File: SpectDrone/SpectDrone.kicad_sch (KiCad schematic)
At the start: 128 parts, among them J1 Conn_02x03_Counter_Clockwise, J1-1 Conn_01x04_Male, J1-2 Conn_01x04_Male, J1V0-1 Conn_01x01_Male, J2 GPS, J3 Barrel_Jack, J3V1-1 Conn_01x01_Male, J3V3 Conn_01x01_Male, J4 BME280, J5 RFShield_OnePiece, J5-1 BNO055-1, J5-2 BNO055-2, J5V3-1 Conn_01x01_Male, J5V3-2 Conn_01x01_Male, Q1 FDN340P, Q2 FDN340P, SW0 SW_Push, SW1 SW_Push, SW10 SW_Push, SW2 SW_Push, SW3 SW_Push, SW4 SW_Push, SW5 SW_Push, SW6 SW_Push, SW7 SW_Push, SW8 SW_Push, SW9 SW_Push, U1 C12666MA, U10 TXS0102DCUR, U11 PCA9306DC, U12 AD799x, U2 C12666MA, U3 LM7805_TO220, U4 MCP112-450E/TO, U5 MCP112-450E/TO, U6 LM7805_TO220, U7 Teensy4.0

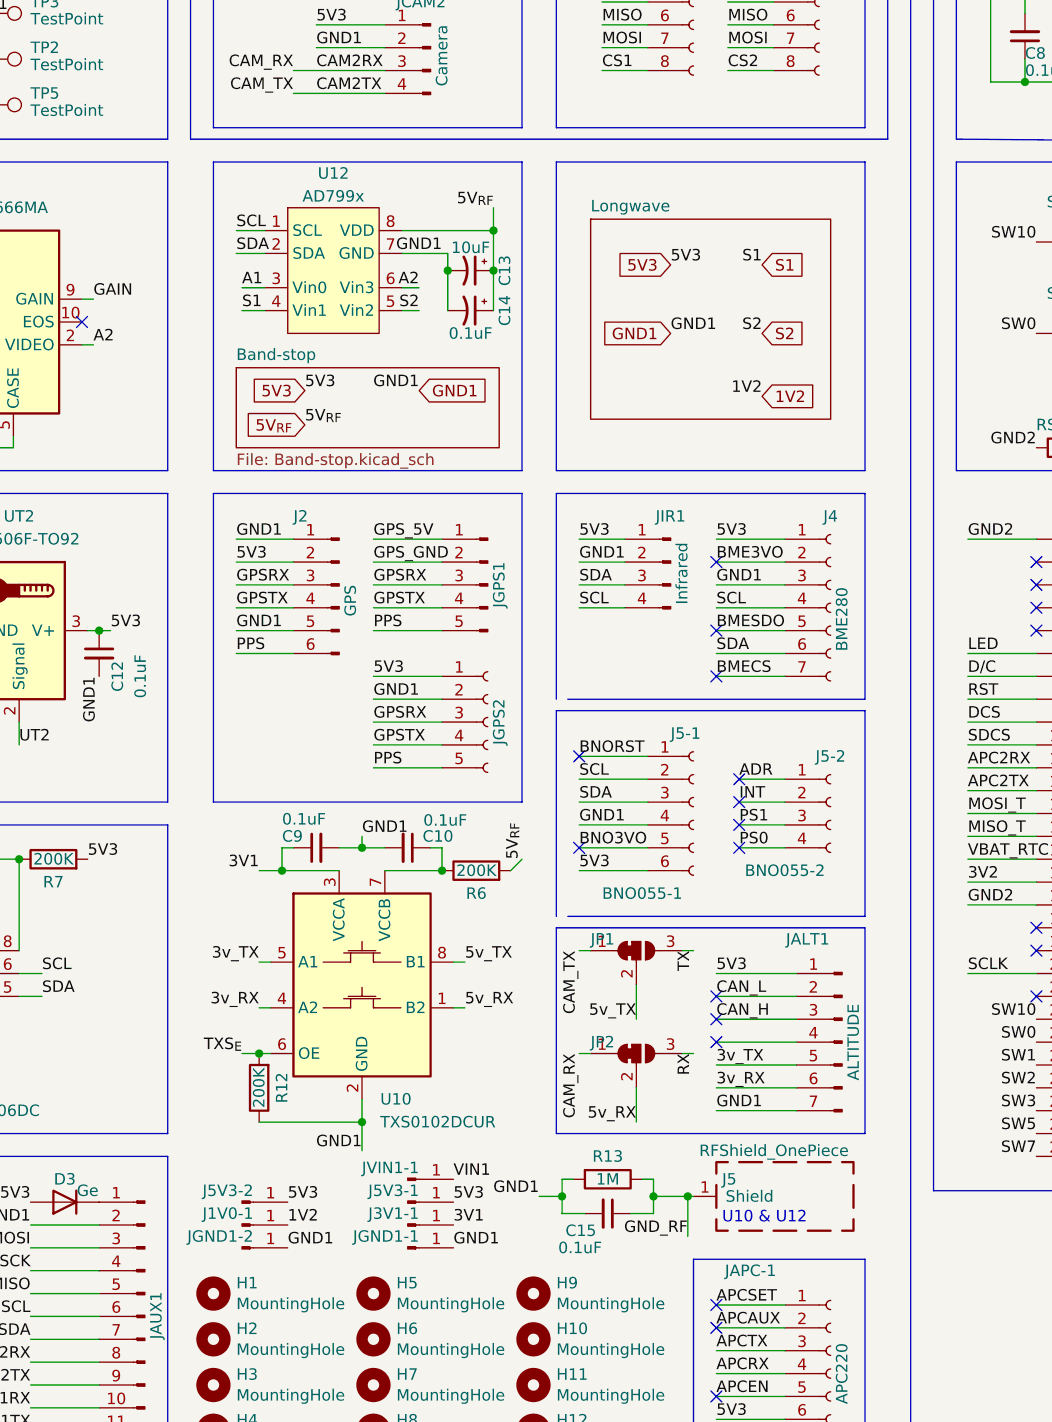
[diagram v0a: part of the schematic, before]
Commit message: SpectDrone Development
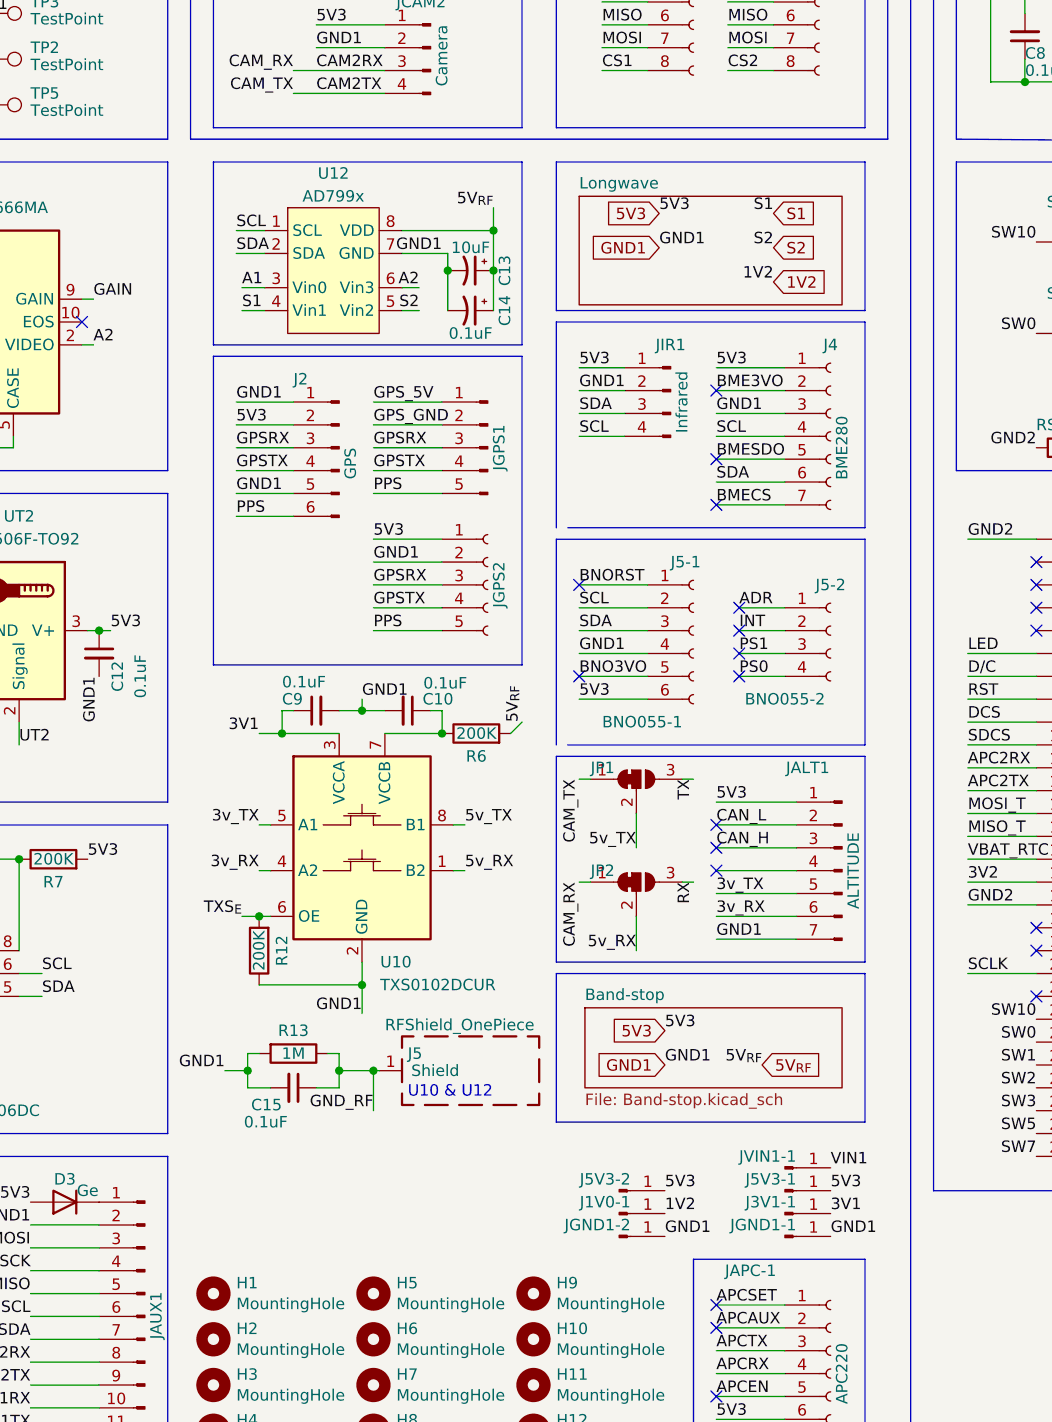
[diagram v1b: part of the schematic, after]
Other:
- moved on the sheet: C10, C15, C9, J1V0-1, J2, J3V1-1, J4, J5, J5-1, J5-2, J5V3-1, J5V3-2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
